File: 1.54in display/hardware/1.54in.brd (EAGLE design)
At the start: 44.5 x 38.1 mm, 69 parts, among them J2 MICRO-SD_CARD_SOCKETPUSH-PUSH, Q1 310mA/60V/1.6Ω, U2 3.3V, U4 23K640

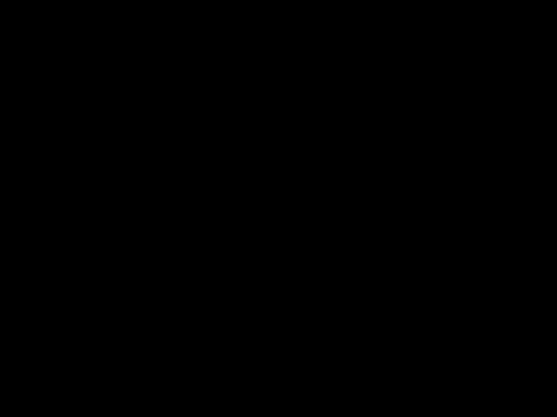
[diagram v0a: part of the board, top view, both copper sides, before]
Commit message: documentation
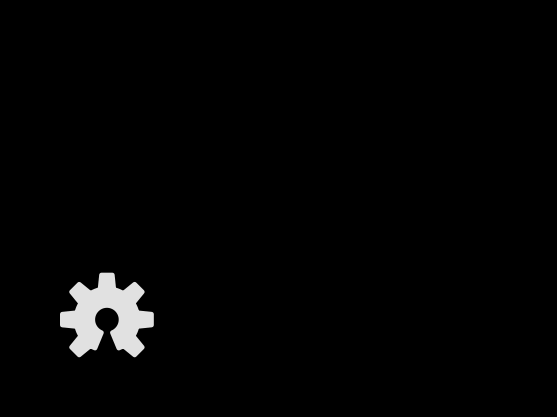
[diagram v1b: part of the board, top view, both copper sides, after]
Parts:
- added LOGO1: OSHW-LOGOS, SparkFun-Aesthetics:OSHW-LOGO-S
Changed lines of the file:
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@@
 <element name="U$32" library="buzzard_labels (33)" package="5V10" value="" x="5.334" y="6.35" rot="MR0"/>
 <element name="U$12" library="buzzard_labels (33)" package="3SPI0" value="" x="29.972" y="4.445"/>
+<element name="LOGO1" library="SparkFun-Aesthetics" package="OSHW-LOGO-S" value="OSHW-LOGOS" x="-16.51" y="-13.97"/>
 </elements>
 <signals>

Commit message: add datasheets
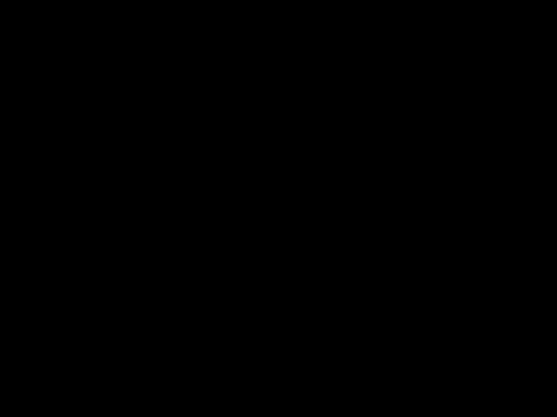
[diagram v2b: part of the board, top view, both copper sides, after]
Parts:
- removed U$2: (no value), SparkFun-Aesthetics:OSHW-LOGO-S
- moved LOGO1 60.5 mm to (41.4, 3.68)
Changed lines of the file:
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@@
 </element>
 <element name="U4" library="SparkFun-IC-Memory" package="SOIC-8" value="23K640" x="19.05" y="4.445" rot="R90"/>
-<element name="U$2" library="SparkFun-Aesthetics" package="OSHW-LOGO-S" value="" x="41.402" y="3.683"/>
 <element name="U$3" library="SparkFun-IC-Comms" package="UFDFN-20" value="TXB0108DQSR" x="8.763" y="17.526" rot="R90">
 <attribute name="PROD_ID" value="IC-12292" x="8.763" y="17.526" size="1.778" layer="27" rot="R90" display="off"/>
@@
 <element name="U$32" library="buzzard_labels (33)" package="5V10" value="" x="5.334" y="6.35" rot="MR0"/>
 <element name="U$12" library="buzzard_labels (33)" package="3SPI0" value="" x="29.972" y="4.445"/>
-<element name="LOGO1" library="SparkFun-Aesthetics" package="OSHW-LOGO-S" value="OSHW-LOGOS" x="-16.51" y="-13.97"/>
+<element name="LOGO1" library="SparkFun-Aesthetics" package="OSHW-LOGO-S" value="OSHW-LOGOS" x="41.402" y="3.683"/>
 </elements>
 <signals>
